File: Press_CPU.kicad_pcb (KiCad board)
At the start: 2 copper layers, 40 x 35 mm, 96 parts, among them J2 2-215079-0, U1 APM32F405RGT6, U10 LMV321, U11 LMV321, U12 FM25W256, U13 LMV321, U14 LMV321, U15 LMV321, U16 LMV321, U2 LM2594HVM-3.3, Y1 CSTCE8M00G55A-R0

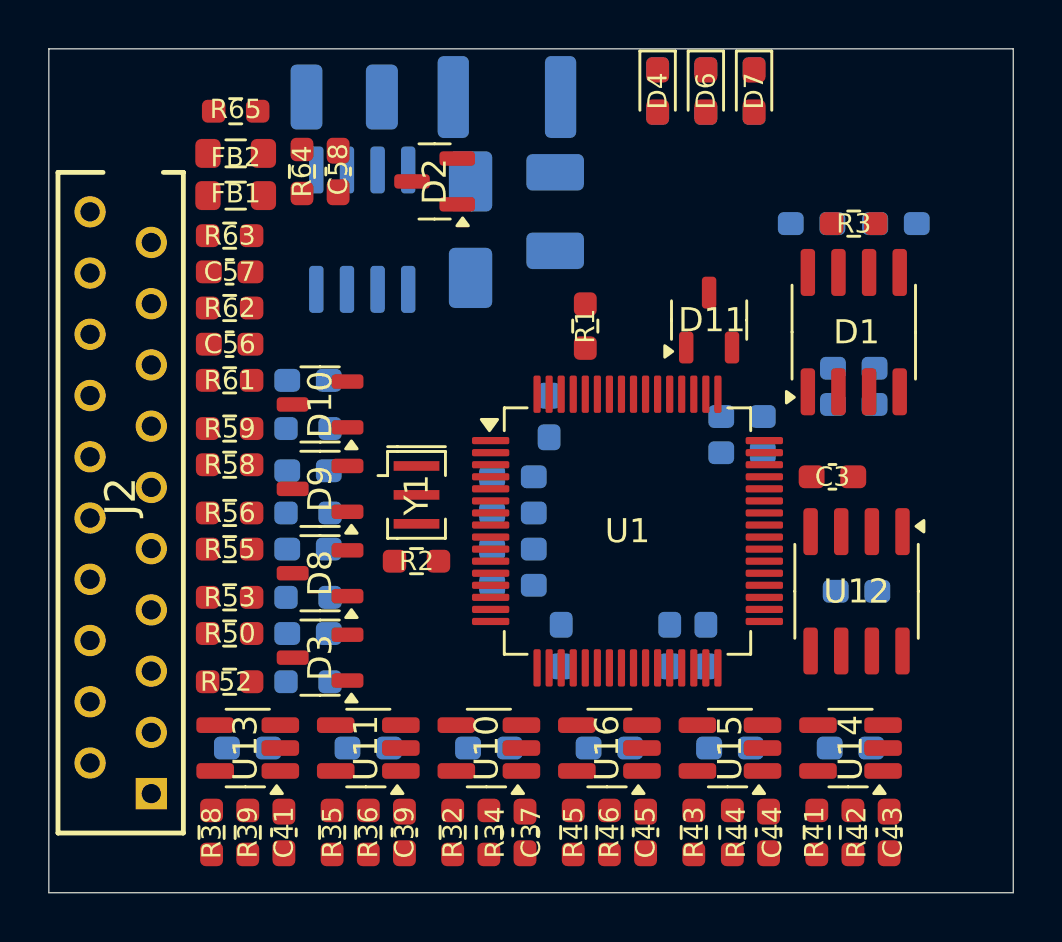
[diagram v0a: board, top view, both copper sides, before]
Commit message: VER1.0: добавил гребенку
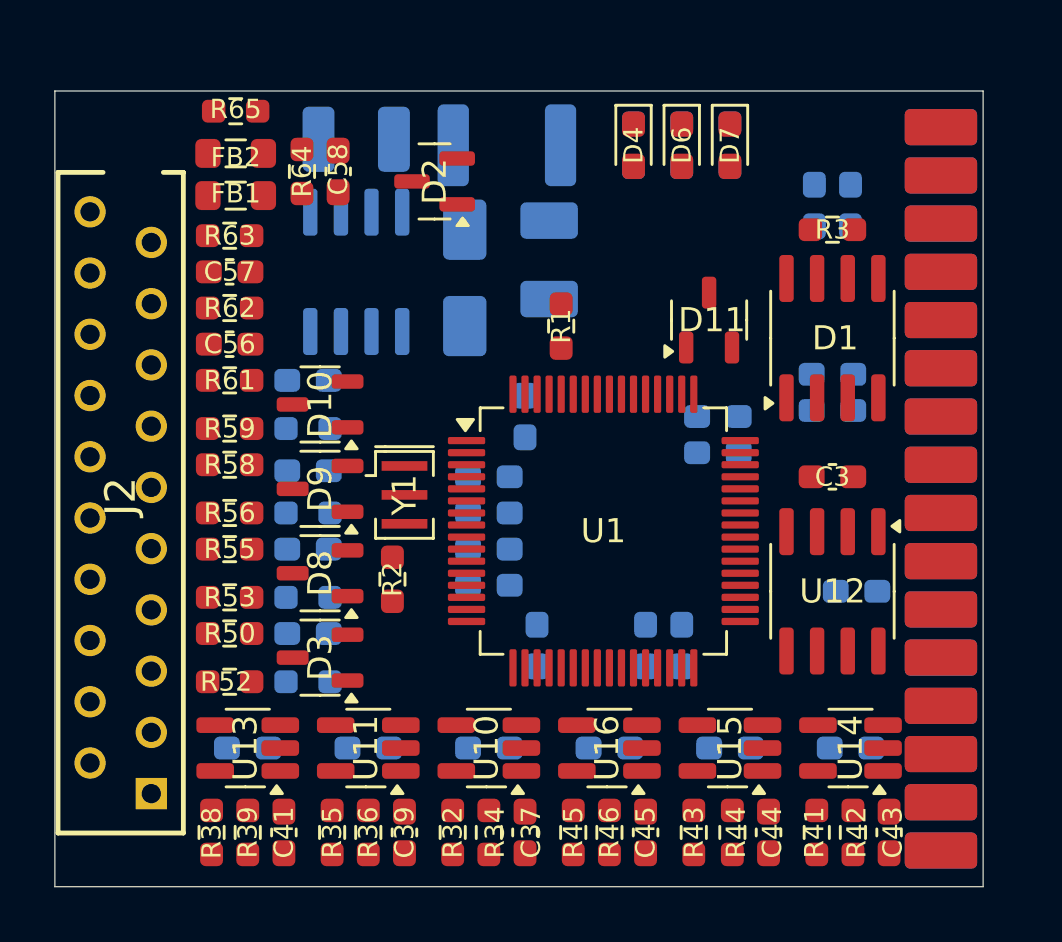
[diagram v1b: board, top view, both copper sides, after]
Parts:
- added J3: Conn_01x16, PLD_my:PLD16_2.0mm, B.Cu at (163.2, 84.0)
- added J4: Conn_01x16, PLD_my:PLD16_2.0mm, F.Cu at (163.2, 114.0)
- moved D4 2.46 mm to (150.5, 84.8)
- moved D6 2.46 mm to (152.5, 84.8)
- moved D7 2.46 mm to (154.5, 84.8)
- moved R4 2.46 mm to (150.5, 84.8)
- moved R5 2.46 mm to (154.5, 84.8)
- moved R6 2.46 mm to (152.5, 84.8)
- moved C10 2.03 mm to (159.5, 87.2), turned to 90 degrees
- moved C19 2.02 mm to (147.0, 89.5)
- moved D5 2.01 mm to (143.5, 90.2)
- moved L1 2.00 mm to (145.2, 84.8)
- moved C17 1.82 mm to (139.0, 84.5)
- moved U2 1.77 mm to (139.0, 90.0)
- moved R2 1.25 mm to (140.5, 102.8), turned to 90 degrees
- moved C1 1.00 mm to (152.5, 105.5)
- moved C12 1.00 mm to (144.5, 103.0)
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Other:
- board size 40 x 35 mm -> 38.5 x 33 mm
- copper layers 2 -> 4
